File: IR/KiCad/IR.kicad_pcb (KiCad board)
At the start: 2 copper layers, 17.8 x 15.2 mm, 4 parts, among them J1 Conn_01x06

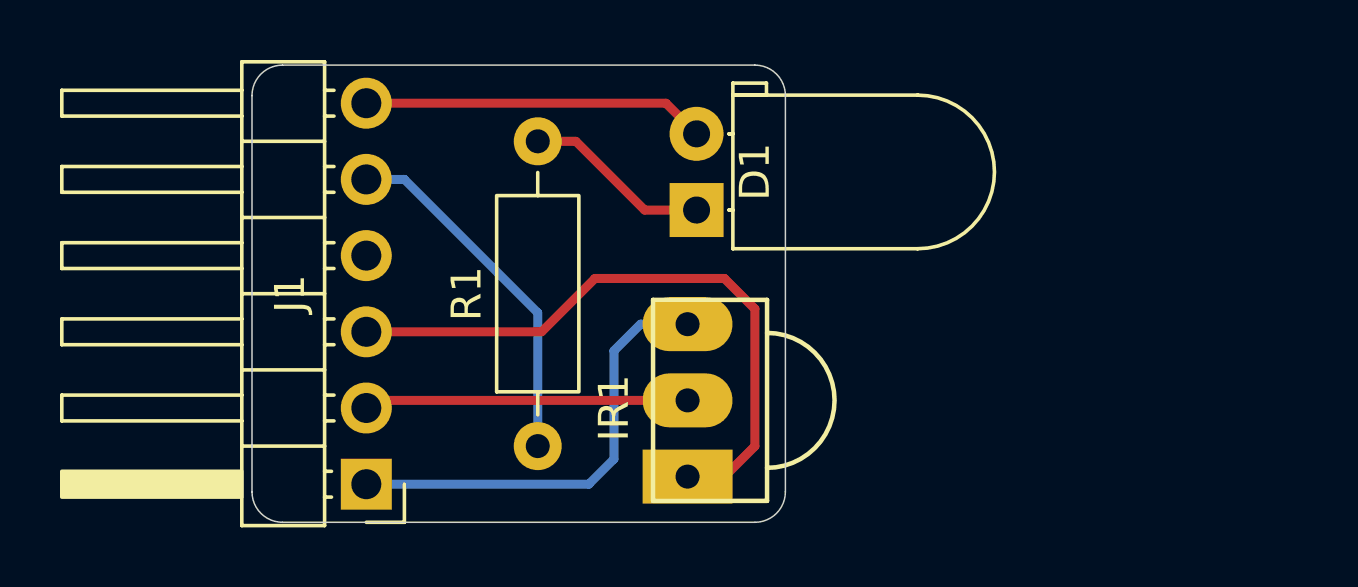
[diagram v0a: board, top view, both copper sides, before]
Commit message: Deployed e8763eb with MkDocs version: 1.6.0
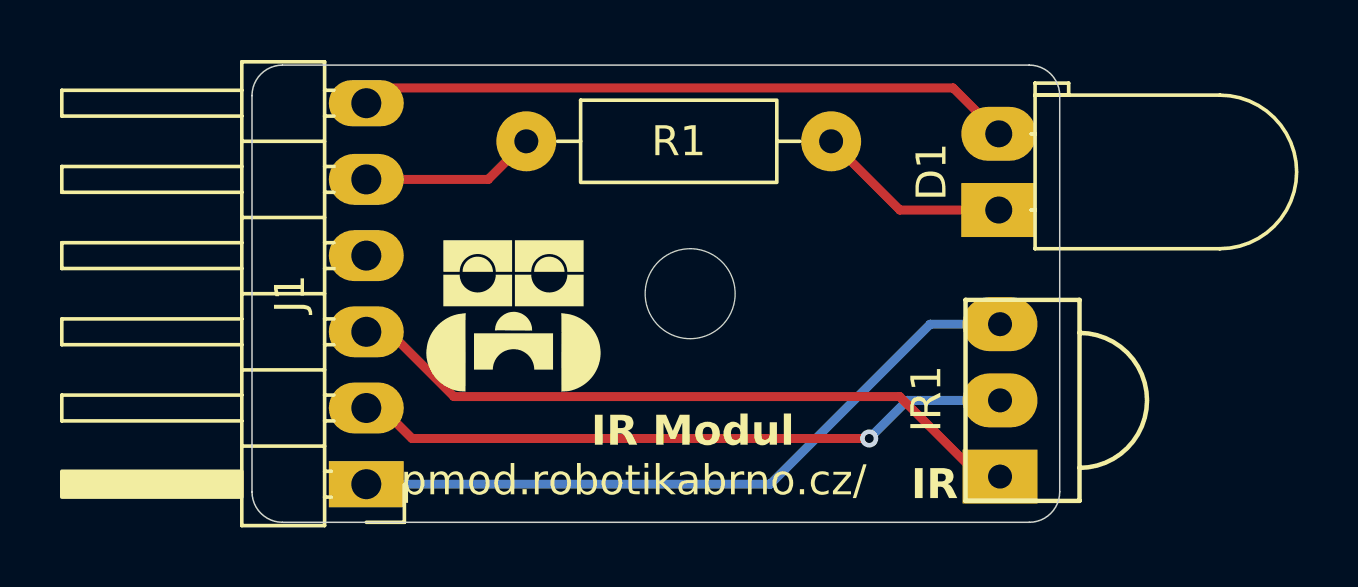
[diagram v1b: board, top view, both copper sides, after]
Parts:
- added REF**: MountingHole_3mm, MountingHole:MountingHole_3mm, F.Cu at (85.7, 50.8)
- moved IR1 10.4 mm to (96.1, 54.4)
- moved R1 10.2 mm to (80.3, 45.7), turned to 0 degrees
- moved D1 10.1 mm to (96.0, 48.0)
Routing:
- net GND: track 10.8 -> 22.9 mm, vias 0 -> 1
- net CLK: track 11.4 -> 21.9 mm
- net +3.3V: track 15.0 -> 23.8 mm
- net TX: track 12.0 -> 5.86 mm
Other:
- board size 17.8 x 15.2 mm -> 26.9 x 15.2 mm
- board text added: "IR"
- board text added: "IR Modul"
- board text added: "pmod.robotikabrno.cz/"
